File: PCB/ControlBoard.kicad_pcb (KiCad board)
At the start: 2 copper layers, 15 parts, among them J1 Conn_01x02, J2 Conn_01x12, SW1 SW_Push, SW2 SW_Push, SW3 SW_Push, U1 Nokia_5510_display_module

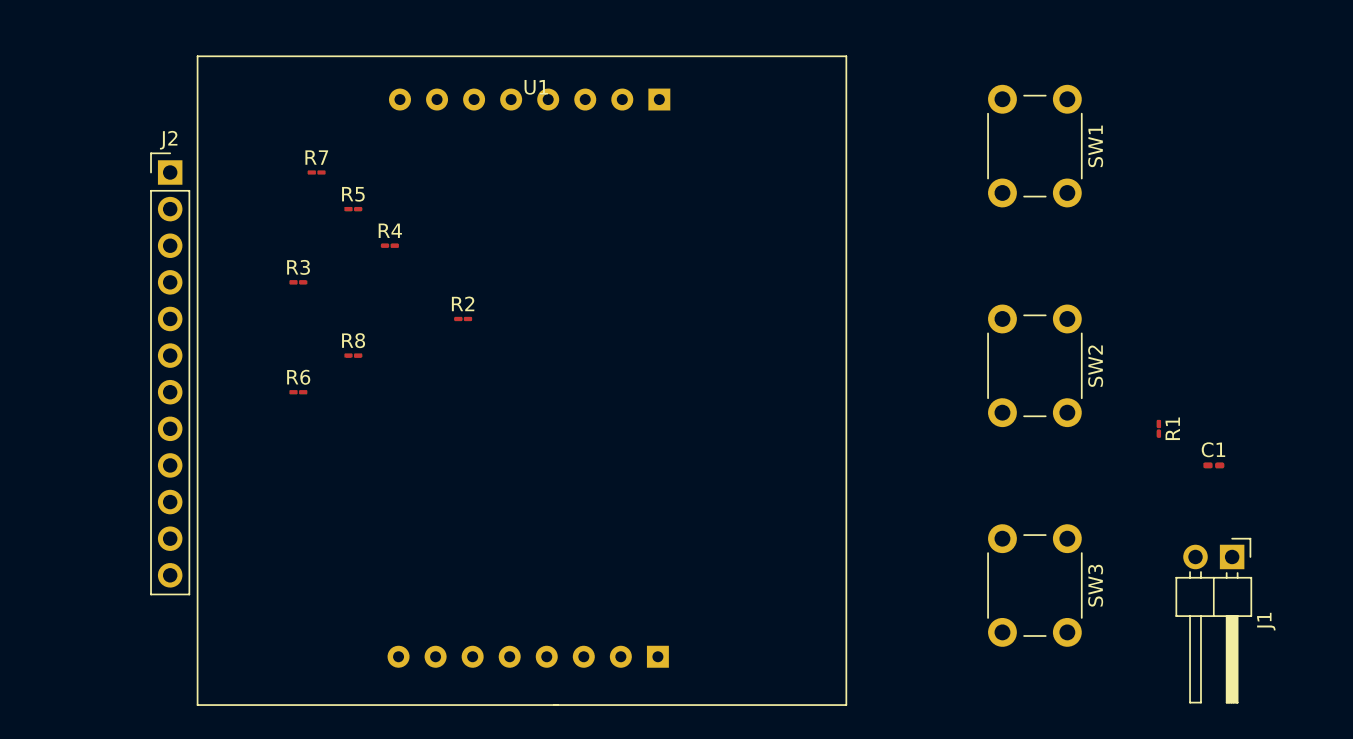
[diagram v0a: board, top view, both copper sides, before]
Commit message: Board done
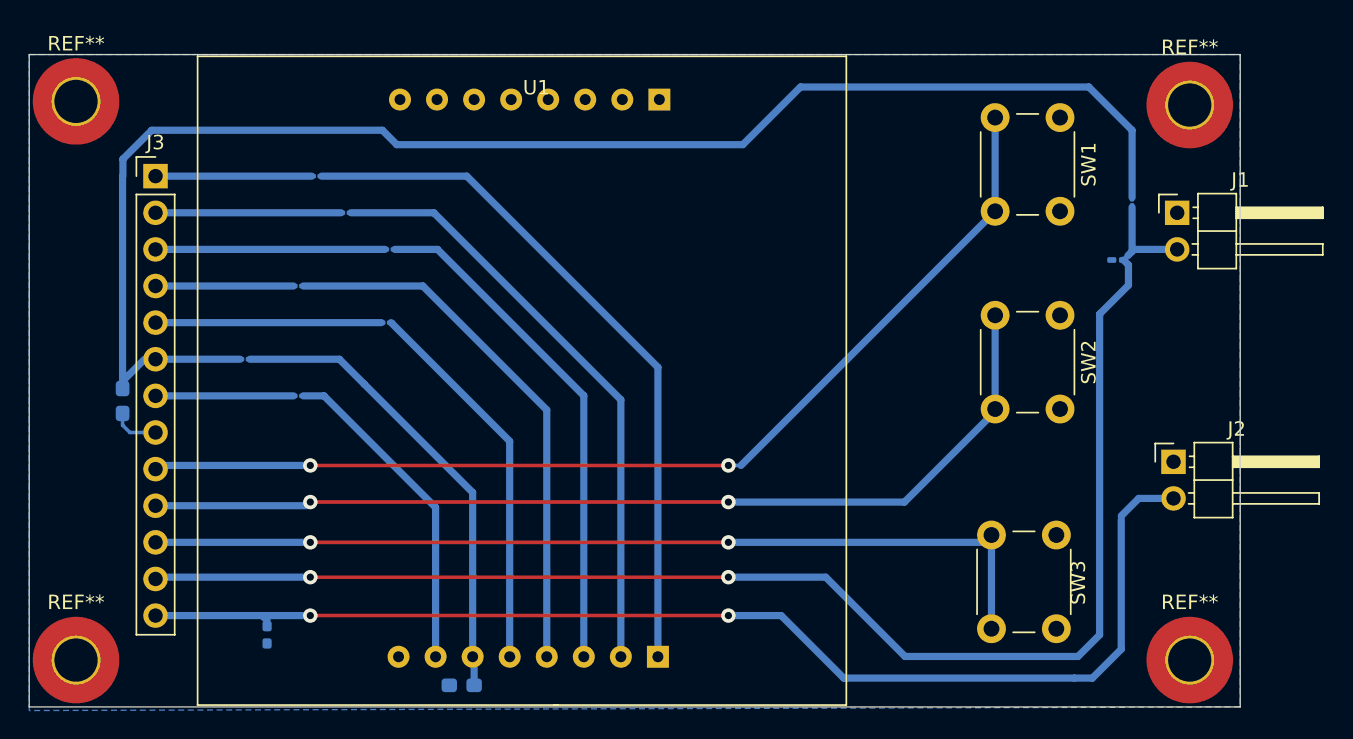
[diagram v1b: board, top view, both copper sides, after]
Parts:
- added C2: 100u, Capacitor_SMD:C_0603_1608Metric_Pad1.08x0.95mm_HandSolder, B.Cu at (101.5, 110.5)
- added C3: 100u, Capacitor_SMD:C_0603_1608Metric_Pad1.08x0.95mm_HandSolder, B.Cu at (78.0, 90.8)
- added J3: Conn_01x13, Connector_PinHeader_2.54mm:PinHeader_1x13_P2.54mm_Vertical, F.Cu at (80.3, 75.2)
- added R9: 10k, Resistor_SMD:R_0402_1005Metric_Pad0.72x0.64mm_HandSolder, B.Cu at (88.0, 107.0)
- added REF**: MountingHole_3mm_Pad_TopOnly, MountingHole:MountingHole_3mm_Pad_TopOnly, F.Cu at (74.8, 108.8)
- added REF**: MountingHole_3mm_Pad_TopOnly, MountingHole:MountingHole_3mm_Pad_TopOnly, F.Cu at (74.8, 70.0)
- added REF**: MountingHole_3mm_Pad_TopOnly, MountingHole:MountingHole_3mm_Pad_TopOnly, F.Cu at (152.0, 108.8)
- added REF**: MountingHole_3mm_Pad_TopOnly, MountingHole:MountingHole_3mm_Pad_TopOnly, F.Cu at (152.0, 70.2)
- C1, R1, R2, R3, R4, R5, R6, R7, R8: moved to B.Cu
- J2: value Conn_01x12 -> Conn_01x02; footprint Connector_PinHeader_2.54mm:PinHeader_1x12_P2.54mm_Vertical -> Connector_PinHeader_2.54mm:PinHeader_1x02_P2.54mm_Horizontal
- moved J2 72.4 mm to (150.9, 95.0)
- moved J1 24.2 mm to (151.1, 77.7), turned to 0 degrees
- moved R1 15.8 mm to (148.0, 77.0)
- moved C1 15.7 mm to (147.0, 81.0), turned to 180 degrees
- moved R8 7.52 mm to (86.5, 87.9), turned to 180 degrees
- moved R2 5.34 mm to (96.3, 85.3)
- moved SW1 1.37 mm to (143.0, 71.1)
- moved SW3 0.80 mm to (142.7, 100.1)
- moved R5 0.57 mm to (93.5, 77.7), turned to 180 degrees
- moved SW2 0.57 mm to (143.0, 84.8)
- moved R3 0.25 mm to (90.2, 82.8)
- moved R6 0.25 mm to (90.2, 90.4)
- moved R4 0.25 mm to (96.5, 80.3)
- moved R7 0.25 mm to (91.4, 75.2)
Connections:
- J2 pad 1: RST -> GND
- J2 pad 2: CE -> REL
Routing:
- net +5V: track 0.00 -> 104.0 mm
- net THERM: track 0.00 -> 102.9 mm, vias 0 -> 2
- net REL: track 0.00 -> 83.9 mm, vias 0 -> 2
- net BTN1: track 0.00 -> 72.1 mm, vias 0 -> 2
- net BTN2: track 0.00 -> 67.6 mm, vias 0 -> 2
- net BTN3: track 0.00 -> 64.7 mm, vias 0 -> 2
- net Net-(R7-Pad2): track 0.00 -> 48.9 mm
- net Net-(R5-Pad1): track 0.00 -> 41.9 mm
- net Net-(R3-Pad2): track 0.00 -> 37.6 mm
- net Net-(R4-Pad2): track 0.00 -> 35.4 mm
- net +3V3: track 0.00 -> 32.7 mm
- net Net-(R2-Pad2): track 0.00 -> 26.6 mm
- net Net-(R6-Pad2): track 0.00 -> 22.7 mm
- net DC: track 0.00 -> 15.9 mm
- net CLK: track 0.00 -> 15.7 mm
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- added copper zone on B.Cu, net GND
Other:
- board outline added: 84 x 45.2 mm
- rule trace_min: 0.2 -> 0.5
